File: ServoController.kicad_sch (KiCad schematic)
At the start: 11 parts, among them U1 PCA9685PW,118

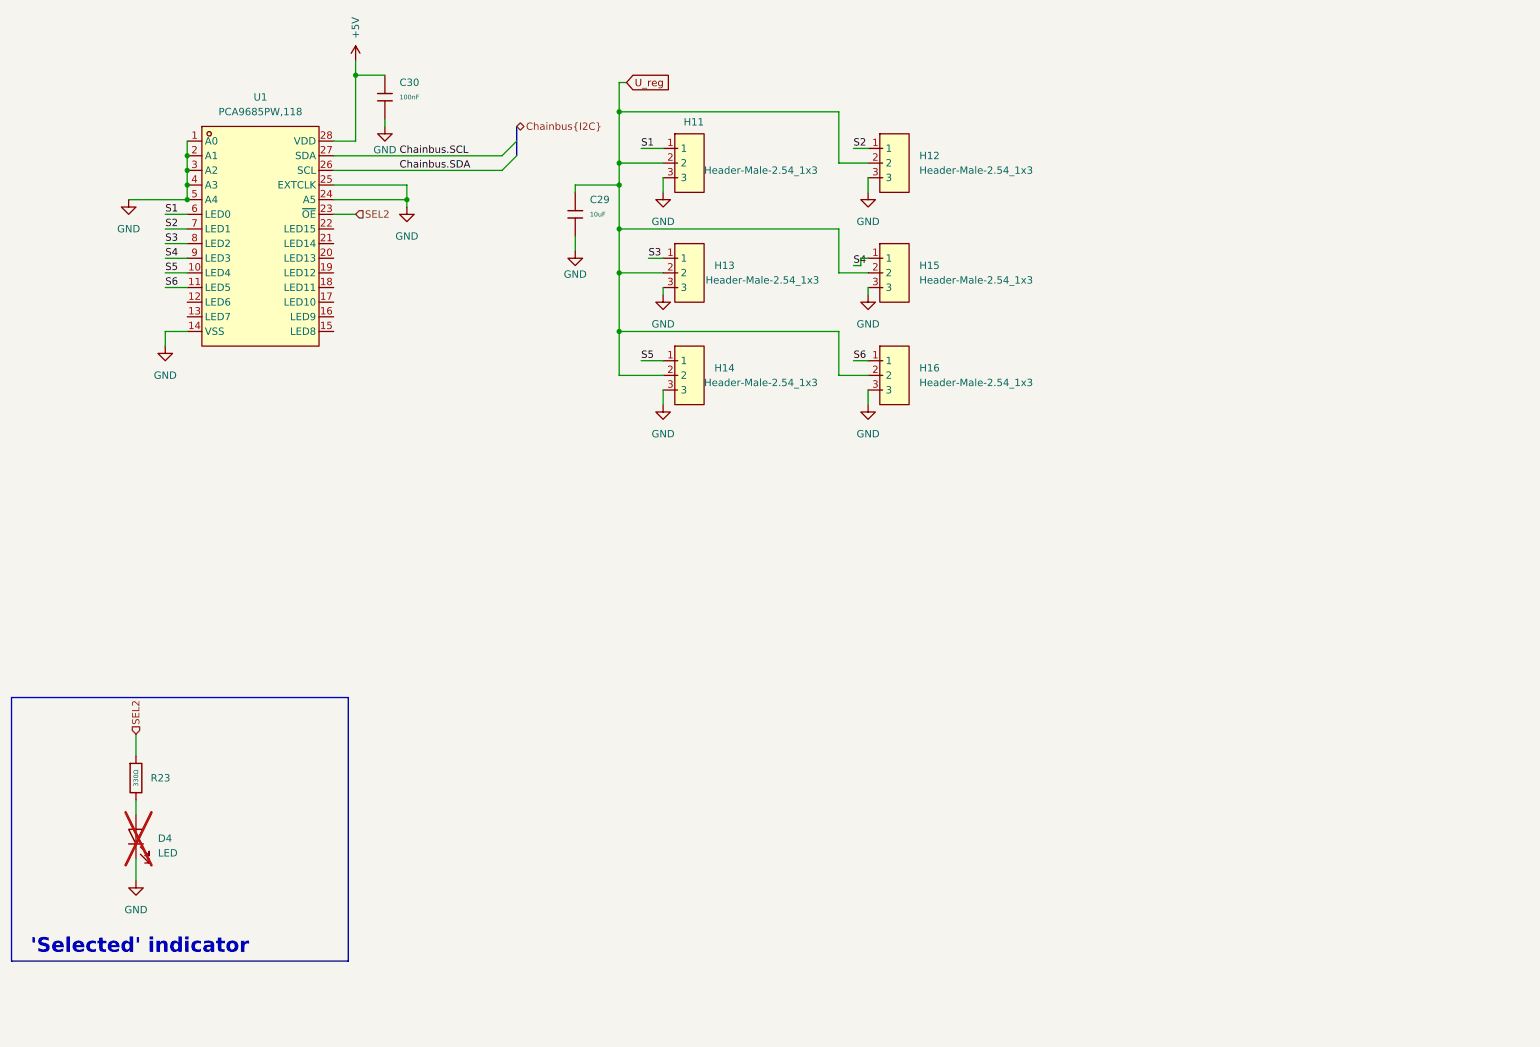
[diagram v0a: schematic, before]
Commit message: polished the schemtic
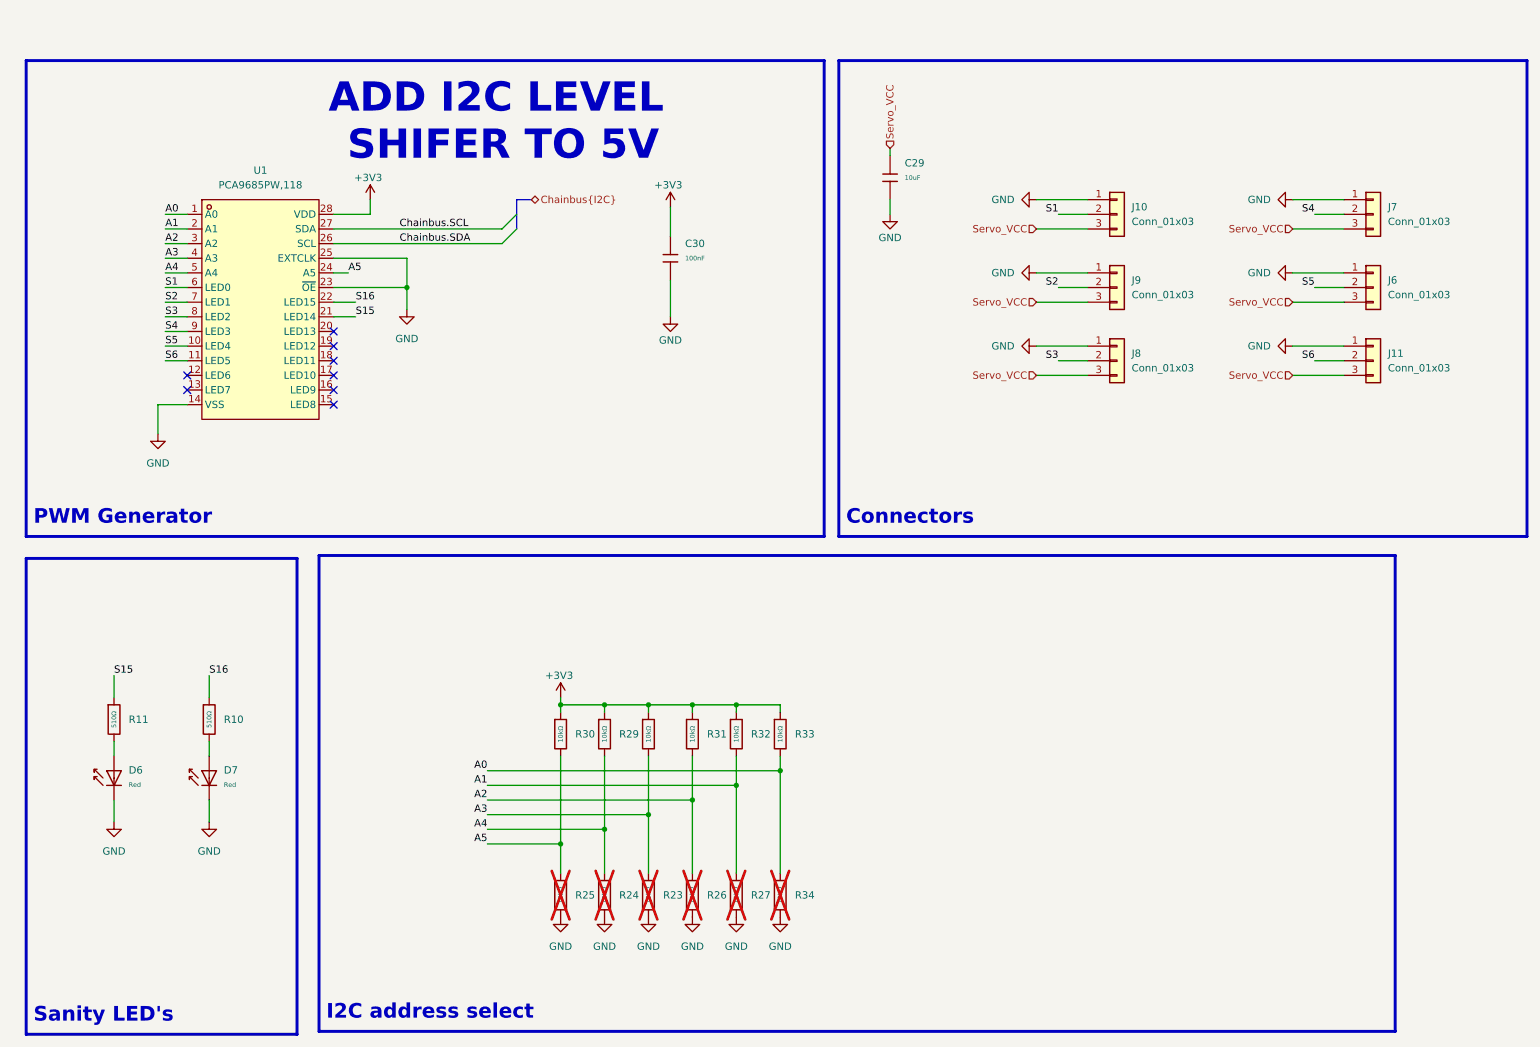
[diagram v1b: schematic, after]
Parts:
- removed D4: LED, LED_SMD:LED_0603_1608Metric, symbol Device:LED
- removed H11, H12, H13, H14, H15, H16: Header-Male-2.54_1x3, easyeda2kicad:HDR-TH_3P-P2.54-V-M-1, symbol SymboleEasyeda2kicad:Header-Male-2.54_1x3
- removed R23: 330Ω, PCM_JLCPCB:R_0402, symbol PCM_JLCPCB-Resistors:0402,330Ω
- added D6, D7: Red, PCM_JLCPCB:D_0603, symbol PCM_JLCPCB-Diodes:LED,0603,Red
- added J10, J11, J6, J7, J8, J9: Conn_01x03, Connector_JST:JST_XH_S3B-XH-A_1x03_P2.50mm_Horizontal, symbol Connector_Generic:Conn_01x03
- added R10, R11: 510Ω, PCM_JLCPCB:R_0402, symbol PCM_JLCPCB-Resistors:0402,510Ω
- added R23, R24, R25, R26, R27, R28, R29, R30, R31, R32, R33, R34: 10kΩ, PCM_JLCPCB:R_0402, symbol PCM_JLCPCB-Resistors:0402,10kΩ
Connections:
- net SEL2 is gone; now on net GND: U1.23 (~{OE})
- net GND: now also D6.1, D7.1, J10.1 (Pin_1), J11.1 (Pin_1), J6.1 (Pin_1), J7.1 (Pin_1), J8.1 (Pin_1), J9.1 (Pin_1), R23.2, R24.2, R25.2, R26.2, R27.2, R34.2; no longer U1.1 (A0), U1.2 (A1), U1.24 (A5), U1.3 (A2), U1.4 (A3), U1.5 (A4)
- net S1: now also J10.2 (Pin_2)
- net S2: now also J9.2 (Pin_2)
- net S3: now also J8.2 (Pin_2)
- net S4: now also J7.2 (Pin_2)
- net S5: now also J6.2 (Pin_2)
- net S6: now also J11.2 (Pin_2)
- net S15: now reaches U1.21 (LED14)
- net S15: now also R11.1
- net S16: now reaches U1.22 (LED15)
- net S16: now also R10.1
- net +5V renamed +3V3
- net +3V3: now also R28.1, R29.1, R30.1, R31.1, R32.1, R33.1
- net U_reg renamed Servo_VCC
- net Servo_VCC: now also J10.3 (Pin_3), J11.3 (Pin_3), J6.3 (Pin_3), J7.3 (Pin_3), J8.3 (Pin_3), J9.3 (Pin_3)
- new net: D6.2, R11.2
- new net: D7.2, R10.2
- new net A0: R33.2, R34.1, U1.1 (A0)
- new net A1: R27.1, R32.2, U1.2 (A1)
- new net A2: R26.1, R31.2, U1.3 (A2)
- new net A3: R23.1, R28.2, U1.4 (A3)
- new net A4: R24.1, R29.2, U1.5 (A4)
- new net A5: R25.1, R30.2, U1.24 (A5)
- no-connect marks 0 -> 8
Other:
- note added: "ADD I2C LEVEL SHIFER TO 5V"
- note added: "Connectors"
- note added: "I2C address select"
- note added: "PWM Generator"
- note added: "Sanity LED's"
- note removed: "'Selected' indicator"
- moved on the sheet: C29, U1
